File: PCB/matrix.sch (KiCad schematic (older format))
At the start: 132 parts, among them K1 GRV, K10 #9, K11 #0, K12 -_, K13 =+, K14 BACK, K15 INS, K16 TAB, K17 Q, K18 W, K19 E, K2 #1, K20 R, K21 T, K22 Y, K23 U, K24 I, K25 O, K26 P, K27 {[, K28 ]}, K29 \\|, K3 #2, K30 DEL, K31 CAPSLOCK, K32 A, K33 S, K34 D, K35 F, K36 G, K37 H, K38 J, K39 K, K4 #3, K40 L, K41 ;:, K42 '\", K43 ENTER, K44 LSHIFT, K45 Z, K46 X, K47 C, K48 V, K49 B, K5 #4, K50 N, K51 M, K52 ,<, K53 .>, K54 /?, K55 RSHIFT, K56 UP, K57 LCTRL, K58 LCOMMAND, K59 LALT, K6 #5, K60 SPACE, K61 RALT, K62 RCOMMAND, K63 RCTRL, K64 LEFT, K65 DOWN, K66 RIGHT, K7 #6, K8 #7, K9 #8

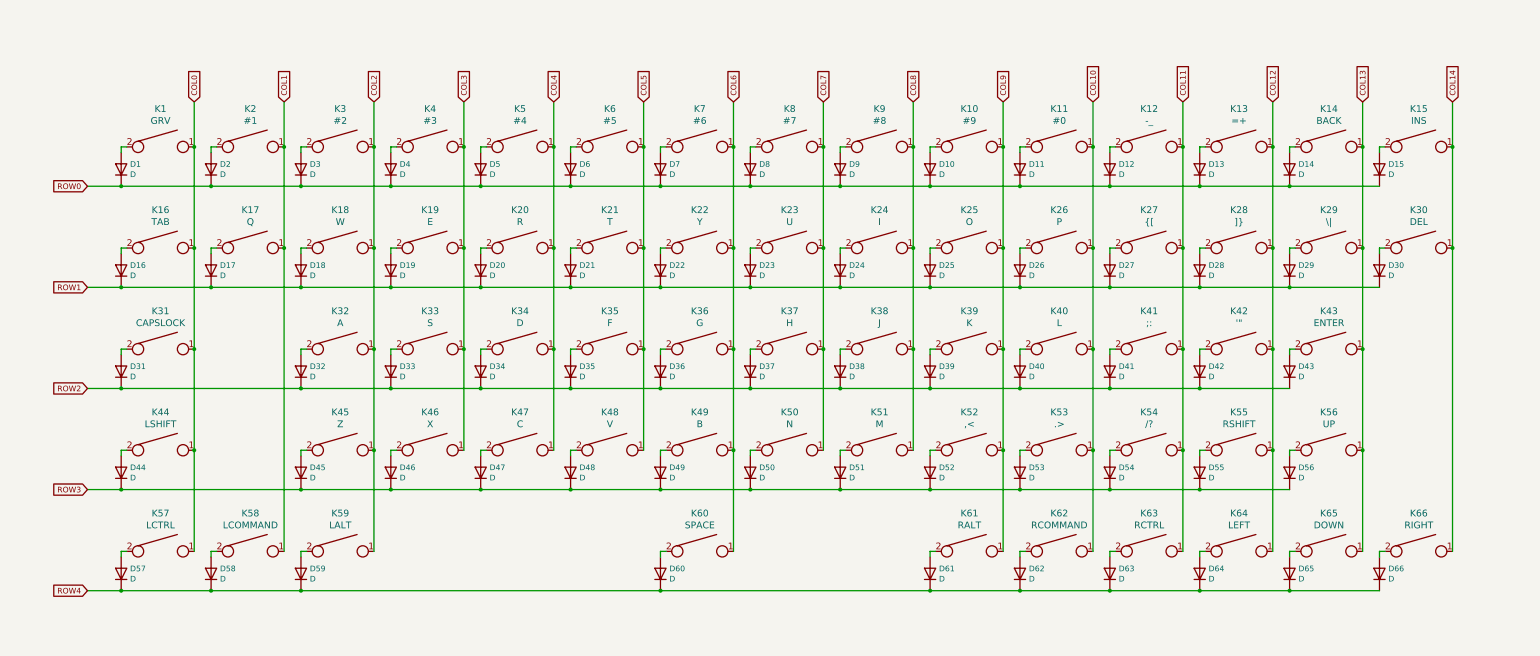
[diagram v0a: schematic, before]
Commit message: Sch Finish
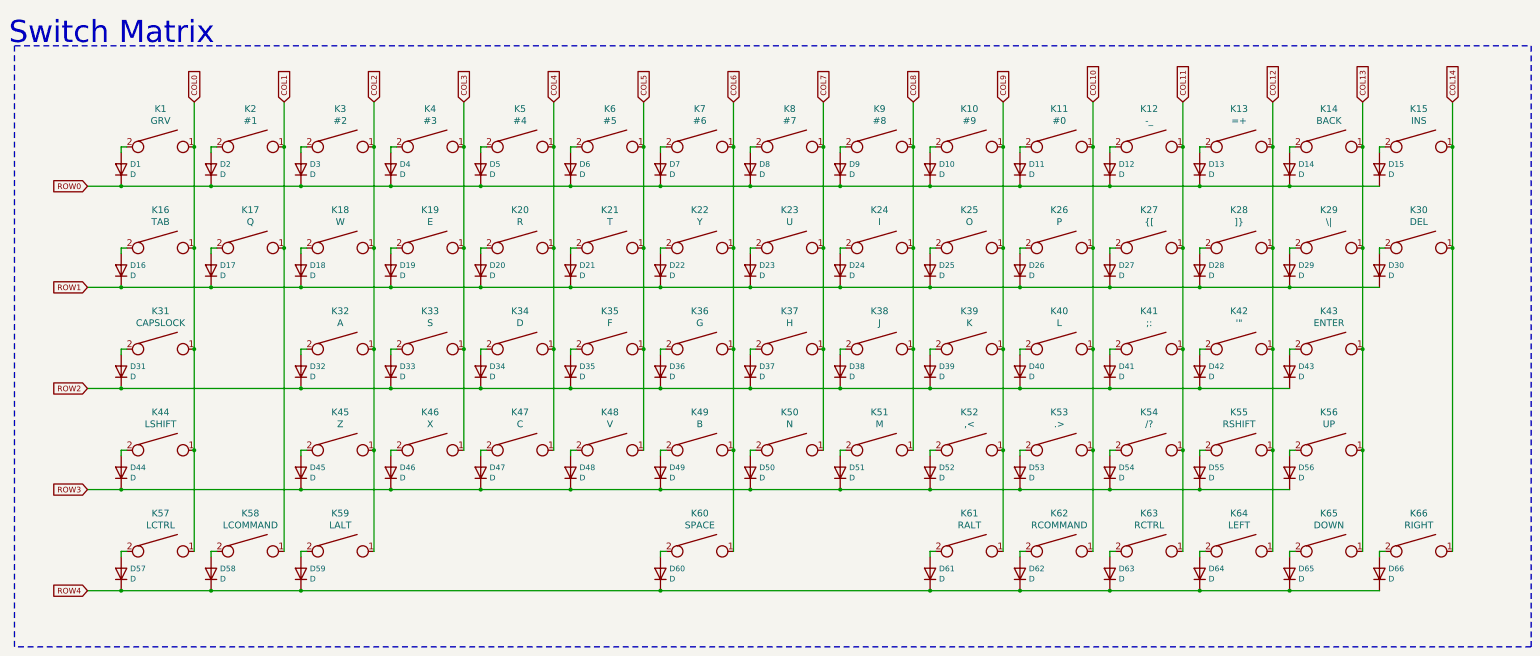
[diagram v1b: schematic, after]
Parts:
- D1, D10, D11, D12, D13, D14, D15, D16, D17, D18, D19, D2, D20, D21, D22, D23, D24, D25, D26, D27, D28, D29, D3, D30, D31, D32, D33, D34, D35, D36, D37, D38, D39, D4, D40, D41, D42, D43, D44, D45, D46, D47, D48, D49, D5, D50, D51, D52, D53, D54, D55, D56, D57, D58, D59, D6, D60, D61, D62, D63, D64, D65, D66, D7, D8, D9: footprint (none) -> Diode_SMD:D_SOD-123
- K1, K10, K11, K12, K13, K15, K17, K18, K19, K2, K20, K21, K22, K23, K24, K25, K26, K27, K28, K3, K30, K32, K33, K34, K35, K36, K37, K38, K39, K4, K40, K41, K42, K45, K46, K47, K48, K49, K5, K50, K51, K52, K53, K54, K56, K58, K6, K64, K65, K66, K7, K8, K9: footprint (none) -> MX_Only:MXOnly-1U-NoLED
- K14: footprint (none) -> MX_Only:MXOnly-2U-NoLED
- K16, K29: footprint (none) -> MX_Only:MXOnly-1.5U-NoLED
- K31: footprint (none) -> MX_Only:MXOnly-1.75U-NoLED
- K43, K44, K55: footprint (none) -> MX_Only:MXOnly-2.25U-NoLED
- K57, K59, K61, K62, K63: footprint (none) -> MX_Only:MXOnly-1.25U-NoLED
- K60: footprint (none) -> MX_Only:MXOnly-6.25U-NoLED
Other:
- note added: "Switch Matrix"

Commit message: Routing 99%
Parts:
- K1, K10, K11, K12, K13, K14, K15, K16, K17, K18, K19, K2, K20, K21, K22, K23, K24, K25, K26, K27, K28, K29, K3, K30, K31, K32, K33, K34, K35, K36, K37, K38, K39, K4, K40, K41, K42, K43, K44, K45, K46, K47, K48, K49, K5, K50, K51, K52, K53, K54, K55, K56, K57, K58, K59, K6, K60, K61, K62, K63, K64, K65, K66, K7, K8, K9: symbol aek67-cache:keyboard_parts_KEYSW -> CrowMiniMk2-rescue:keyboard_parts_KEYSW-aek67-cache

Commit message: Pre Logo add
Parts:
- K1, K10, K11, K12, K13, K15, K17, K18, K19, K2, K20, K21, K22, K23, K24, K25, K26, K27, K28, K3, K30, K32, K33, K34, K35, K36, K37, K38, K39, K4, K40, K41, K42, K45, K46, K47, K48, K49, K5, K50, K51, K52, K53, K54, K56, K58, K6, K64, K65, K66, K7, K8, K9: footprint MX_Only:MXOnly-1U-NoLED -> local:MXOnly-1U-NoLED
- K14: footprint MX_Only:MXOnly-2U-NoLED -> local:MXOnly-2U-NoLED
- K16, K29: footprint MX_Only:MXOnly-1.5U-NoLED -> local:MXOnly-1.5U-NoLED
- K31: footprint MX_Only:MXOnly-1.75U-NoLED -> local:MXOnly-1.75U-NoLED
- K43, K44, K55: footprint MX_Only:MXOnly-2.25U-NoLED -> local:MXOnly-2.25U-NoLED
- K57, K59, K61, K62, K63: footprint MX_Only:MXOnly-1.25U-NoLED -> local:MXOnly-1.25U-NoLED
- K60: footprint MX_Only:MXOnly-6.25U-NoLED -> local:MXOnly-6.25U-NoLED

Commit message: Save1.2.2
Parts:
- D1, D10, D11, D12, D13, D14, D15, D16, D17, D18, D19, D2, D20, D21, D22, D23, D24, D25, D26, D27, D28, D29, D3, D30, D31, D32, D33, D34, D35, D36, D37, D38, D39, D4, D40, D41, D42, D43, D44, D45, D46, D47, D48, D49, D5, D50, D51, D52, D53, D54, D55, D56, D57, D58, D59, D6, D60, D61, D62, D63, D64, D65, D66, D7, D8, D9: LCSC (none) -> C77978
